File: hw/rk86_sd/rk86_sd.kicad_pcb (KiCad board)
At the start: 2 copper layers, 30.5 x 50.2 mm, 16 parts, among them J1 PC Interface, J2 AVR ISP, J3 Micro_SD_Card_Det_Hirose_DM3AT, U1 ATmega328-A, U2 AMS1117-3.3, U3 4050

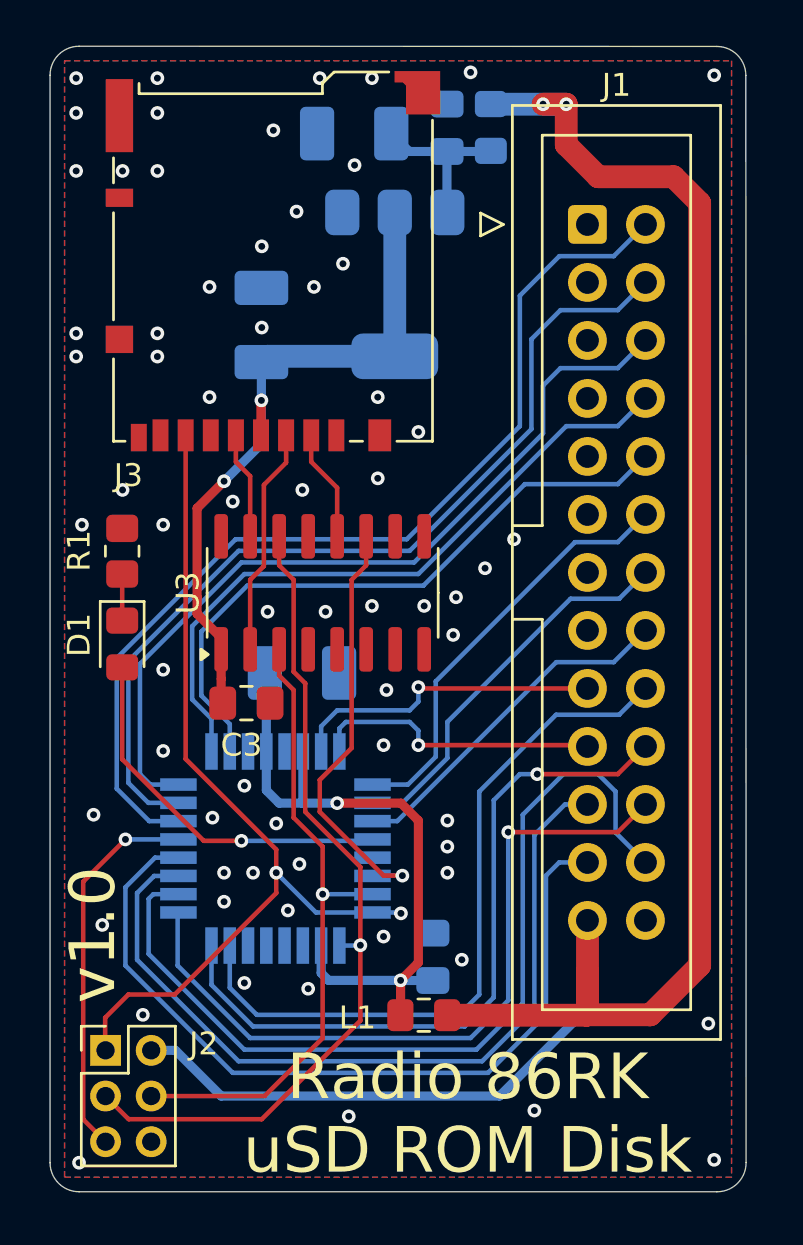
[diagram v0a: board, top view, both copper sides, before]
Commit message: small pcb edition
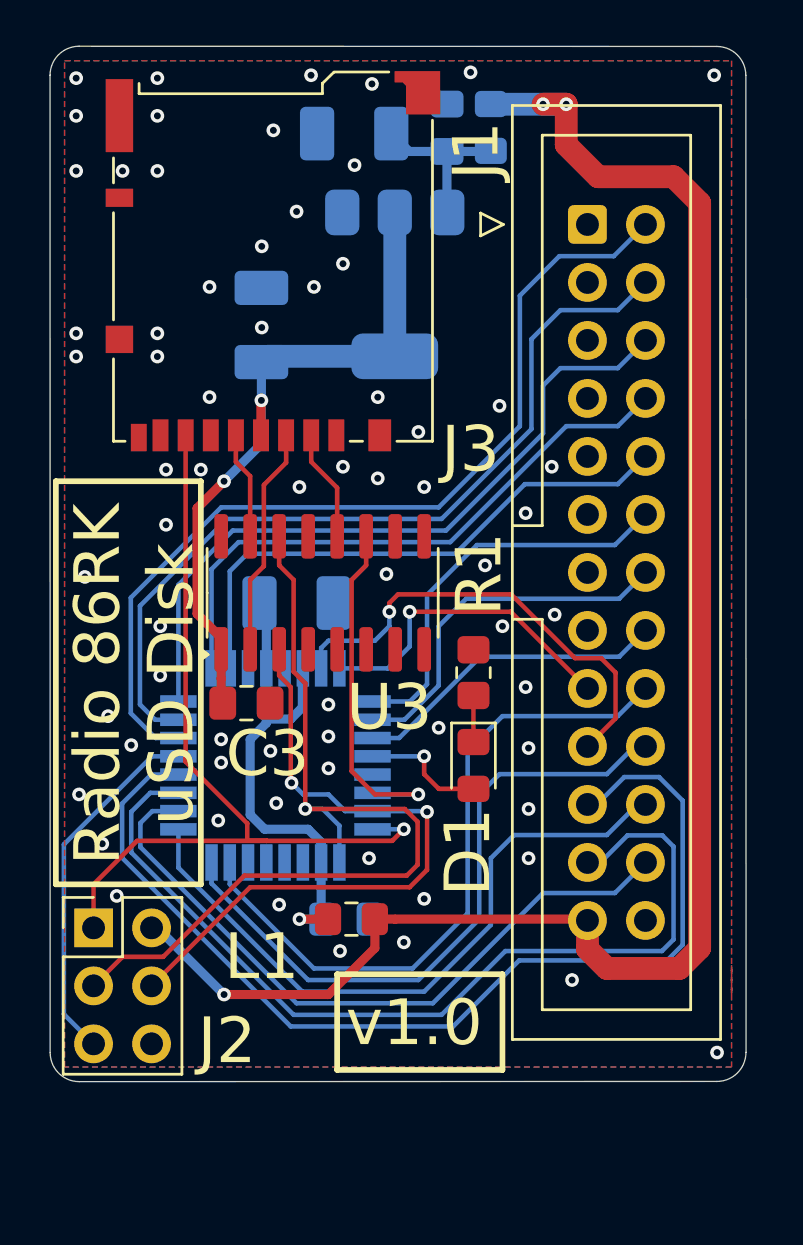
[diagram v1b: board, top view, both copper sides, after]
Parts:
- J2: footprint Connector_PinHeader_2.00mm:PinHeader_2x03_P2.00mm_Vertical -> Connector_PinHeader_2.54mm:PinHeader_2x03_P2.54mm_Vertical
- moved D1 16.3 mm to (183.0, 67.7)
- moved R1 16.3 mm to (183.0, 63.6)
- moved J2 5.39 mm to (166.4, 74.8)
- moved L1 5.27 mm to (177.7, 74.4)
- moved C1 4.13 mm to (177.4, 74.4), turned to 0 degrees
- moved U1 3.64 mm to (174.3, 67.7)
- moved C6 3.07 mm to (175.3, 60.6)
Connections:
- U1 pad 27: /BUS_A5 -> /BUS_A4
- U1 pad 28: /BUS_A4 -> /BUS_A5
- U1 pad 7: /BUS_A7 -> /BUS_A6
- U1 pad 8: /BUS_A6 -> /BUS_A7
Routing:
- net /VCC_5V0: track 89.8 -> 75.0 mm, vias 2 -> 3
- net /LED: track 16.5 -> 5.47 mm
- net /BUS_A5: track 35.7 -> 45.9 mm
- net /BUS_A3: track 39.8 -> 30.4 mm
- net /BUS_A6: track 12.8 -> 20.5 mm
- net Net-(U1-AVCC): track 29.6 -> 23.1 mm, vias 2 -> 1
- net /BUS_A4: track 35.9 -> 40.8 mm
- net /BUS_D2: track 35.9 -> 31.2 mm
- net /BUS_D4: track 28.4 -> 24.5 mm
- net /BUS_D3: track 29.8 -> 26.4 mm
- net /BUS_A2: track 32.7 -> 29.5 mm, vias 1 -> 0
- net /BUS_D0: track 43.4 -> 40.2 mm
- net /BUS_D1: track 39.7 -> 36.6 mm
- net /CARD_SEL: track 19.0 -> 15.9 mm
- net /BUS_A1: track 31.6 -> 29.1 mm, vias 1 -> 0
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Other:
- board size 30.5 x 50.2 mm -> 30.5 x 45.3 mm
- board text added: "Radio 86RK uSD Disk"
- board text removed: "Radio 86RK uSD ROM Disk"
